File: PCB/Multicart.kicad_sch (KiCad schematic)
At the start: 46 parts, among them J1 MODULE, SW1 BACK, SW2 NEXT, U1 74HC00, U2 74LS573, U3 SST39SF040, U4 SST39SF040, U5 SST39SF040, U6 SA39-11SRWA, U7 MAX810, U8 AT89C2051-12P, Y1 3.6864MHz

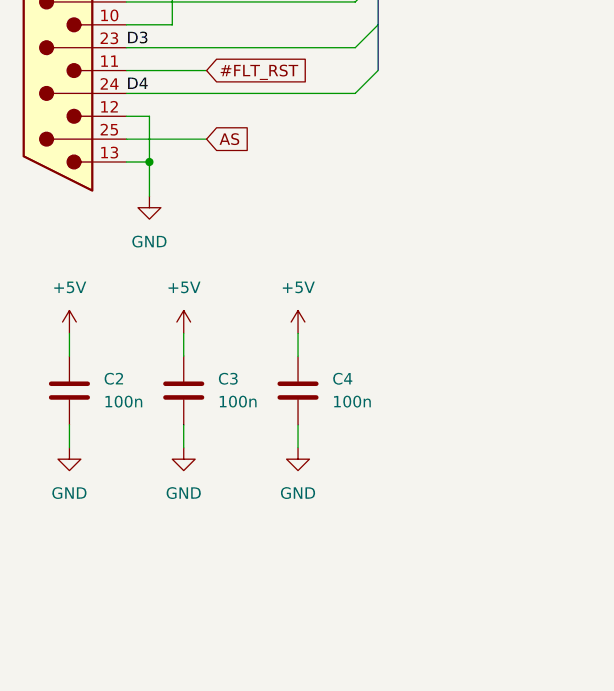
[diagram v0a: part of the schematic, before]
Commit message: Update for production
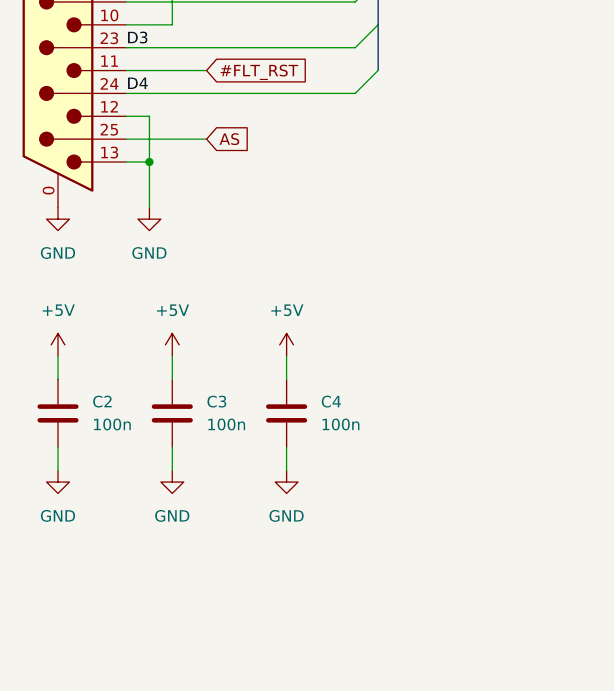
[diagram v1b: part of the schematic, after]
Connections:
- net GND: now also J1.0
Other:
- moved on the sheet: C2, C3, C4
